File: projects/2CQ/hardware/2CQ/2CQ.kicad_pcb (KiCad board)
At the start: 4 copper layers, 17 parts, among them SW1 TOGGLE_ON-ON, U1 ES_DAISY_PATCH_SM_REV1

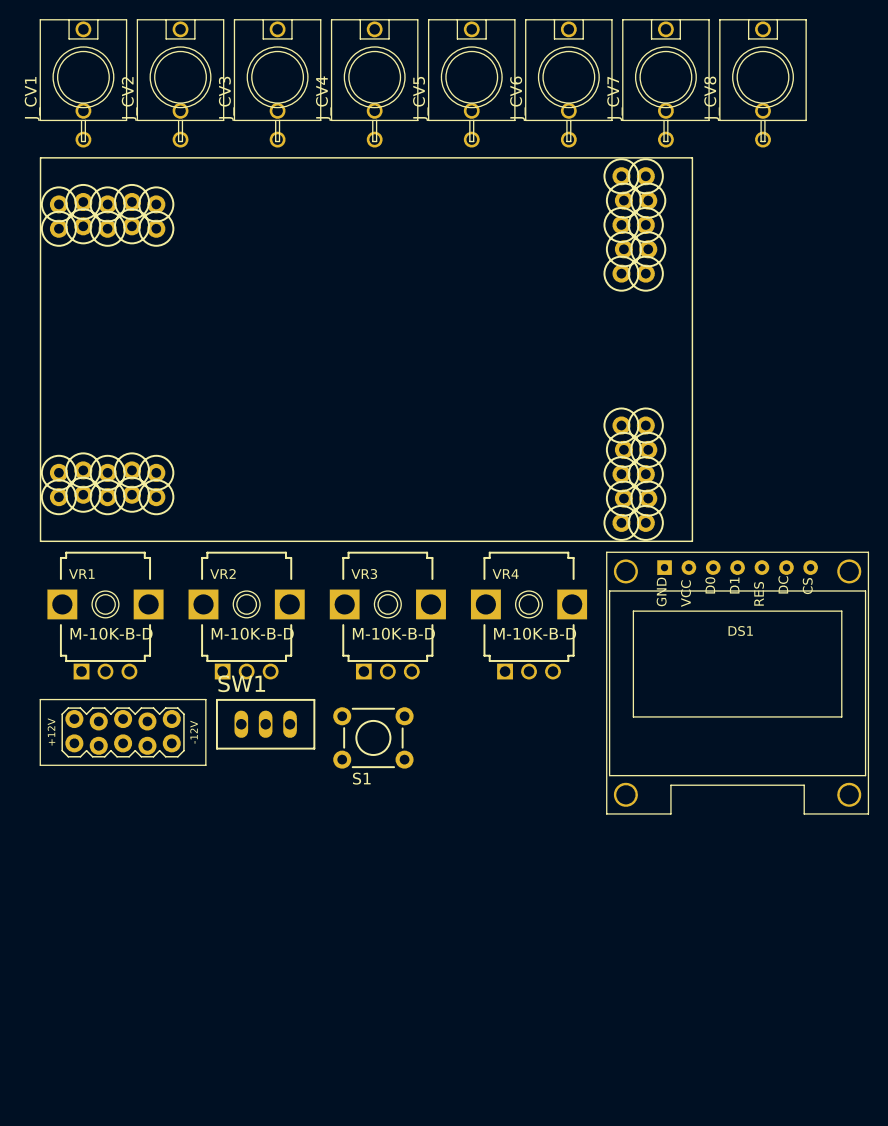
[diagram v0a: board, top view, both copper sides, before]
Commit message: Added 3d models and updated PCB
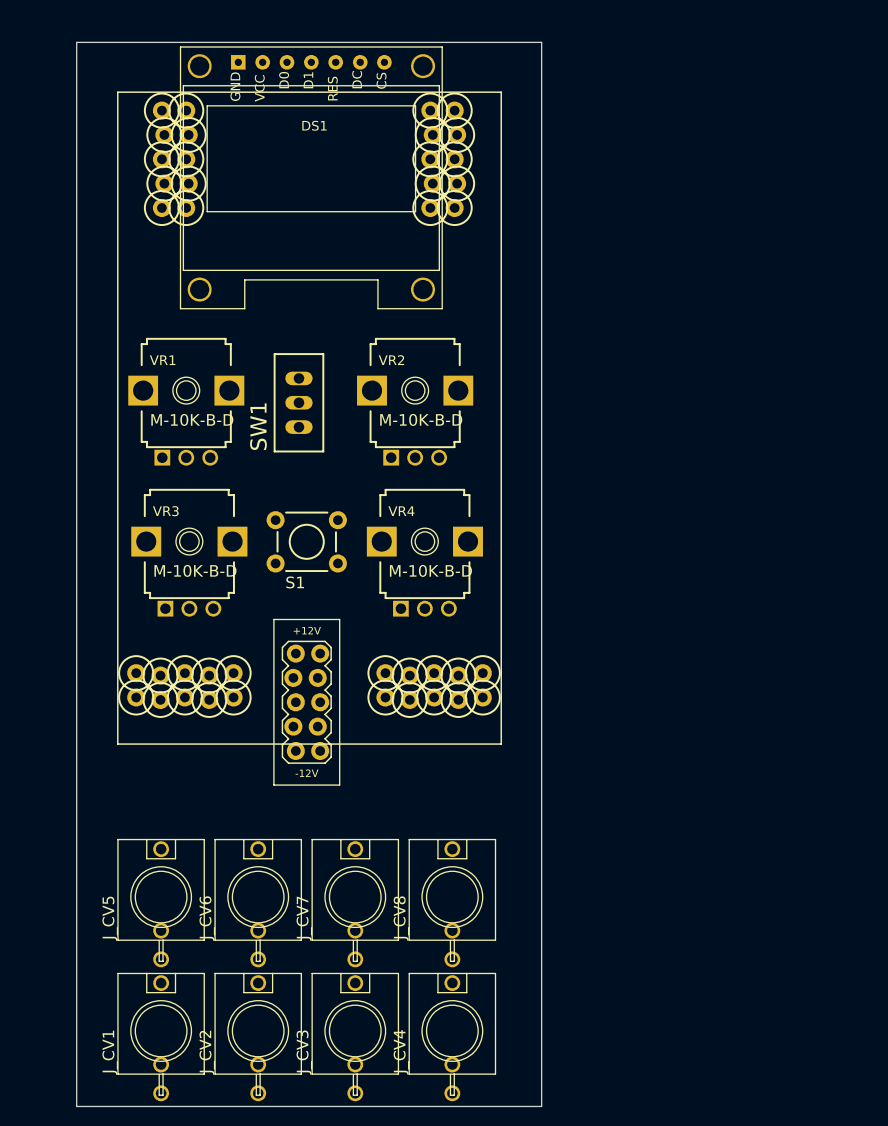
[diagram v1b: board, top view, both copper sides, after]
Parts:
- moved J_CV1 99.8 mm to (82.4, 147.6)
- moved J_CV2 99.8 mm to (92.5, 147.6)
- moved J_CV3 99.8 mm to (102.6, 147.6)
- moved J_CV4 99.8 mm to (112.8, 147.6)
- moved J_CV7 91.4 mm to (102.6, 133.6)
- moved J_CV5 91.4 mm to (82.4, 133.6)
- moved J_CV6 91.4 mm to (92.5, 133.6)
- moved J_CV8 91.4 mm to (112.8, 133.6)
- moved DS1 69.0 mm to (84.4, 72.2)
- moved SW1 33.7 mm to (96.8, 82.0), turned to 90 degrees
- moved VR2 28.4 mm to (108.9, 80.8)
- moved VR1 23.8 mm to (85.0, 80.8)
- moved VR3 21.7 mm to (85.3, 96.5)
- moved S1 21.6 mm to (97.6, 96.5)
- moved EP1 19.4 mm to (97.6, 113.3), turned to -90 degrees
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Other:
- board outline added: 48.5 x 111 mm
